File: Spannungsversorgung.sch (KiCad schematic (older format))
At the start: 11 parts

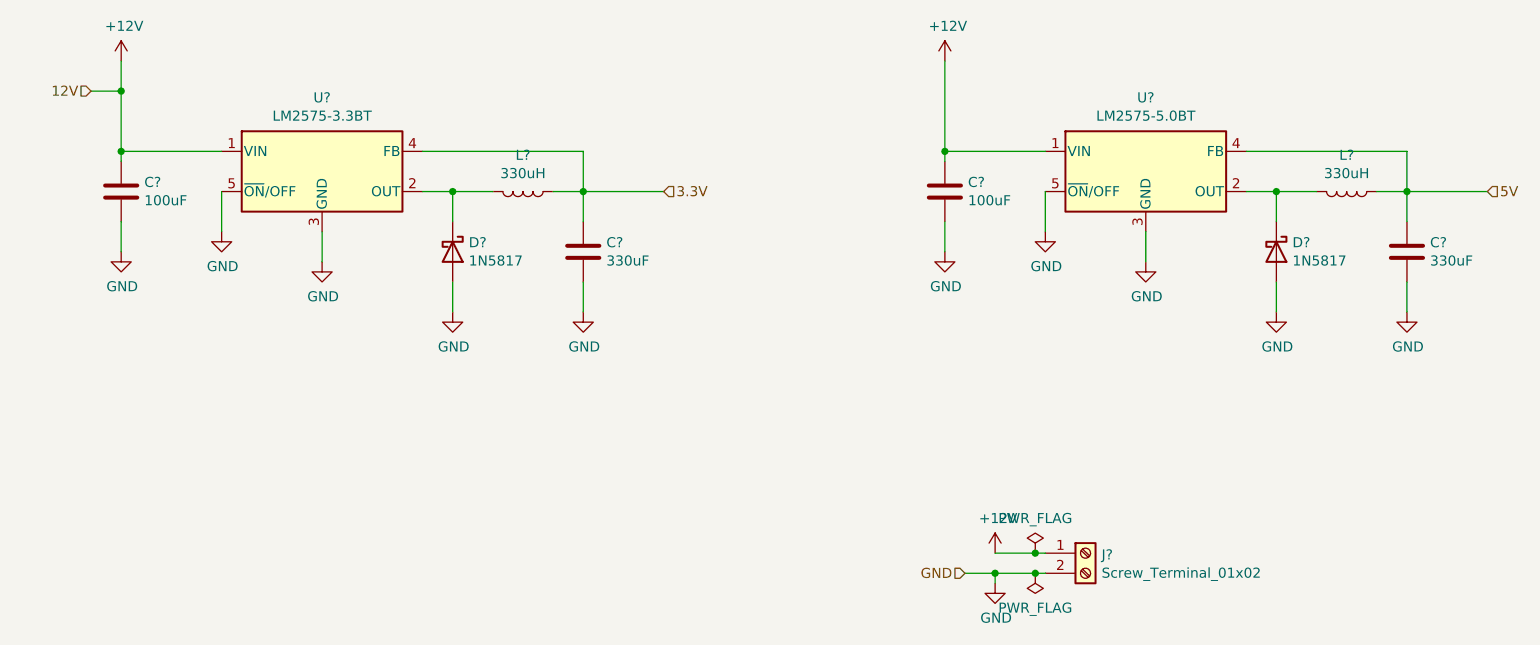
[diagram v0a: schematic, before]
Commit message: i did everithing
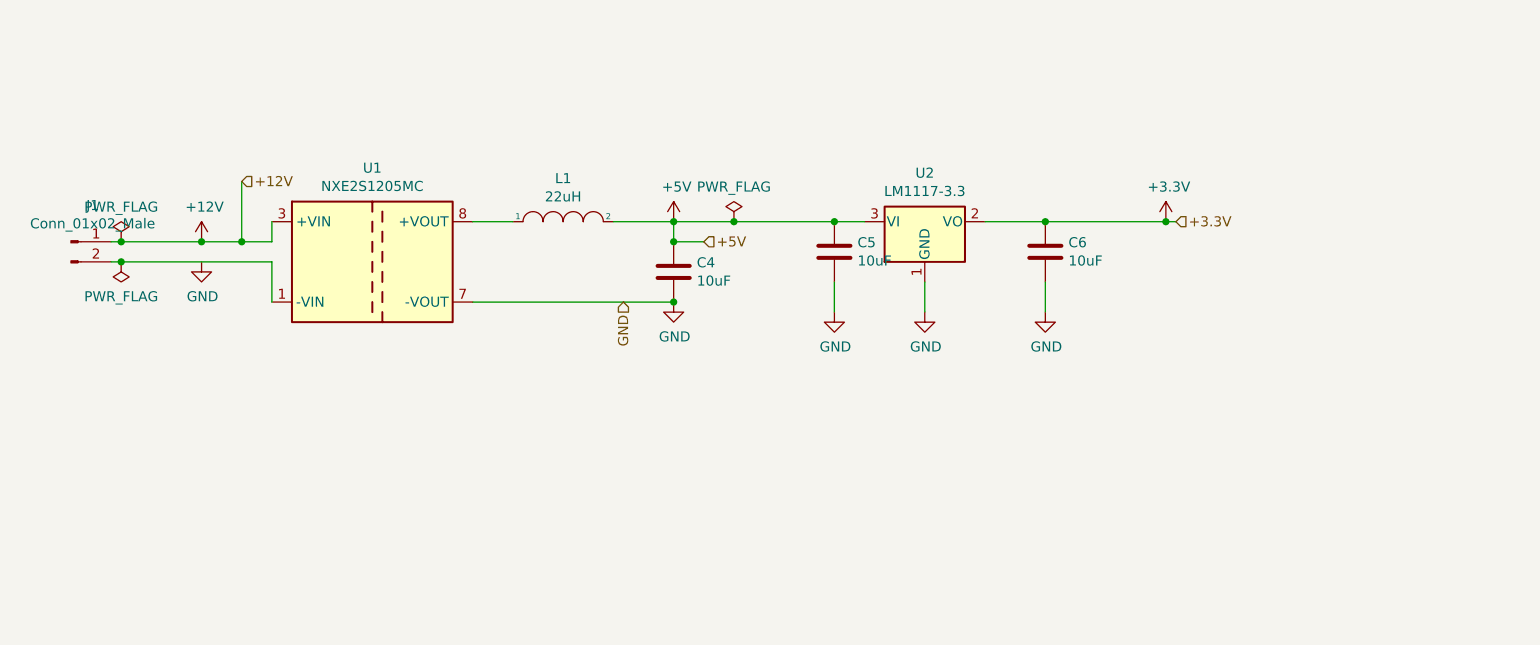
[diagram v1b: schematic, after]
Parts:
- removed C? (x2): 100uF, symbol Device:C
- removed C? (x2): 330uF, symbol Device:C
- removed D? (x2): 1N5817, Diode_THT:D_DO-41_SOD81_P10.16mm_Horizontal, symbol Diode:1N5817
- removed J?: Screw_Terminal_01x02, symbol Connector:Screw_Terminal_01x02
- removed L? (x2): 330uH, symbol Device:L
- removed U?: LM2575-3.3BT, Package_TO_SOT_THT:TO-220-5_Vertical, symbol Regulator_Switching:LM2575-3.3BT
- removed U?: LM2575-5.0BT, Package_TO_SOT_THT:TO-220-5_Vertical, symbol Regulator_Switching:LM2575-5.0BT
- added C4, C5, C6: 10uF, Capacitor_SMD:C_0603_1608Metric_Pad1.08x0.95mm_HandSolder, symbol Device:C
- added J1: Conn_01x02_Male, Connector_Molex:Molex_KK-254_AE-6410-02A_1x02_P2.54mm_Vertical, symbol Connector:Conn_01x02_Male
- added L1: 22uH, EZ-PY32:8200, symbol pspice:INDUCTOR
- added U1: NXE2S1205MC, Converter_DCDC:Converter_DCDC_muRata_NXExSxxxxMC_SMD, symbol Regulator_Switching:NXE2S1205MC
- added U2: LM1117-3.3, Package_TO_SOT_SMD:SOT-223-3_TabPin2, symbol Regulator_Linear:LM1117-3.3
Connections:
- net +12V: now also J1.1 (Pin_1), U1.3 (+VIN)
- net GND: now also C4.2, C5.2, C6.2, U1.7 (-VOUT), U2.1 (GND)
- new net: J1.2 (Pin_2), U1.1 (-VIN)
- new net: L1.1, U1.8 (+VOUT)
- new net +3V3: C6.1, U2.2 (VO)
- new net +5V: C4.1, C5.1, L1.2, U2.3 (VI)
